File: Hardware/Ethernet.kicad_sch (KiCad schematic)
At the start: 37 parts, among them J1 Conn_01x07_Male, J2 Conn_01x04_Male, J3 Conn_01x02_Male, J4 Conn_01x02_Male, J5 Conn_01x02_Male, J6 Conn_01x02_Male, J7 Conn_01x08_Male, J9 QWIIC_Stackable, U1 W5500, Y1 25.000MHz

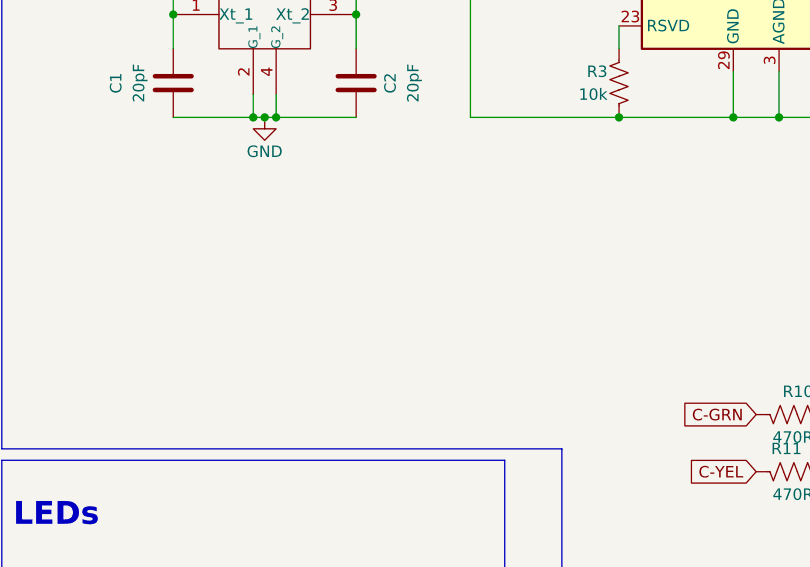
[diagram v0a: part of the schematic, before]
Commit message: More on POE...
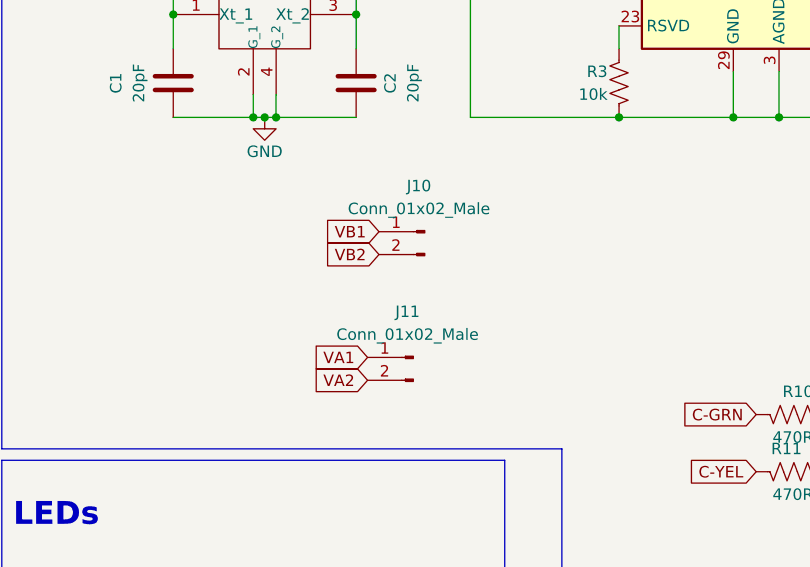
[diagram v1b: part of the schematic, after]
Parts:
- added J10, J11: Conn_01x02_Male, Connector_PinSocket_1.27mm:PinSocket_1x02_P1.27mm_Vertical_SMD_Pin1Right, symbol Connector:Conn_01x02_Male
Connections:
- net VA1: now also J11.1 (Pin_1)
- net VA2: now also J11.2 (Pin_2)
- net VB1: now also J10.1 (Pin_1)
- net VB2: now also J10.2 (Pin_2)
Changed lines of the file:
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@@
+    )
+  )
+  (global_label "VB2" (shape input) (at 157.48 128.27 180) (fields_autoplaced)
+    (effects (font (size 1.27 1.27)) (justify right))
+    (property "Intersheet References" "${INTERSHEET_REFS}" (id 0) (at 151.4988 128.1906 0)
+      (effects (font (size 1.27 1.27)) (justify right) hide)
     )
   )
@@
     )
   )
+  (global_label "VA1" (shape input) (at 156.21 139.7 180) (fields_autoplaced)
+    (effects (font (size 1.27 1.27)) (justify right))
+    (property "Intersheet References" "${INTERSHEET_REFS}" (id 0) (at 150.4102 139.6206 0)
+      (effects (font (size 1.27 1.27)) (justify right) hide)
+    )
+  )
   (global_label "RD+" (shape input) (at 260.35 148.59 0) (fields_autoplaced)
     (effects (font (size 1.27 1.27)) (justify left))
     (property "Intersheet References" "${INTERSHEET_REFS}" (id 0) (at 266.8755 148.5106 0)
       (effects (font (size 1.27 1.27)) (justify left) hide)
+    )
+  )
+  (global_label "VA2" (shape input) (at 156.21 142.24 180) (fields_autoplaced)
+    (effects (font (size 1.27 1.27)) (justify right))
+    (property "Intersheet References" "${INTERSHEET_REFS}" (id 0) (at 150.4102 142.1606 0)
+      (effects (font (size 1.27 1.27)) (justify right) hide)
     )
   )
@@
     (property "Intersheet References" "${INTERSHEET_REFS}" (id 0) (at 268.8107 72.3106 0)
       (effects (font (size 1.27 1.27)) (justify left) hide)
+    )
+  )
+  (global_label "VB1" (shape input) (at 157.48 125.73 180) (fields_autoplaced)
+    (effects (font (size 1.27 1.27)) (justify right))
+    (property "Intersheet References" "${INTERSHEET_REFS}" (id 0) (at 151.4988 125.6506 0)
+      (effects (font (size 1.27 1.27)) (justify right) hide)
     )
   )
@@
     (property "Type" "Tantalum" (id 5) (at 193.04 33.02 0))
     (property "LCSC" "C127946" (id 4) (at 199.39 33.02 0)
+      (effects (font (size 1.27 1.27)) hide)
+    )
+    (pin "1")
+    (pin "2")
+  )
+  (symbol (lib_id "Connector:Conn_01x02_Male") (at 161.29 139.7 0) (mirror y) (unit 1)
+    (in_bom no) (on_board yes)
+    (property "Reference" "J11" (id 0) (at 160.655 134.62 0))
+    (property "Value" "Conn_01x02_Male" (id 1) (at 160.655 137.16 0))
+    (property "Footprint" "Connector_PinSocket_1.27mm:PinSocket_1x02_P1.27mm_Vertical_SMD_Pin1Right" (id 2) (at 161.29 139.7 0)
+      (effects (font (size 1.27 1.27)) hide)
+    )
+    (property "Datasheet" "~" (id 3) (at 161.29 139.7 0)
       (effects (font (size 1.27 1.27)) hide)
     )
@@
     (pin "1")
   )
+  (symbol (lib_id "Connector:Conn_01x02_Male") (at 162.56 125.73 0) (mirror y) (unit 1)
+    (in_bom no) (on_board yes)
+    (property "Reference" "J10" (id 0) (at 161.925 120.65 0))
+    (property "Value" "Conn_01x02_Male" (id 1) (at 161.925 123.19 0))
+    (property "Footprint" "Connector_PinSocket_1.27mm:PinSocket_1x02_P1.27mm_Vertical_SMD_Pin1Right" (id 2) (at 162.56 125.73 0)
+      (effects (font (size 1.27 1.27)) hide)
+    )
+    (property "Datasheet" "~" (id 3) (at 162.56 125.73 0)
+      (effects (font (size 1.27 1.27)) hide)
+    )
+    (pin "1")
+    (pin "2")
+  )
   (symbol (lib_id "Connector:Conn_01x07_Male") (at 72.39 35.56 0) (unit 1)
     (in_bom no) (on_board no)
@@
       (reference "J9") (unit 1) (value "QWIIC_Stackable") (footprint "Tinker:QWIIC_Stack_II")
     )
+    (path "/a064da1d-e50b-4d46-9902-76208c1e200e"
+      (reference "J10") (unit 1) (value "Conn_01x02_Male") (footprint "Connector_PinSocket_1.27mm:PinSocket_1x02_P1.27mm_Vertical_SMD_Pin1Right")
+    )
+    (path "/504ed9d0-691d-452d-b516-7f09cf7e2eae"
+      (reference "J11") (unit 1) (value "Conn_01x02_Male") (footprint "Connector_PinSocket_1.27mm:PinSocket_1x02_P1.27mm_Vertical_SMD_Pin1Right")
+    )
     (path "/99ba0a0f-3edd-4786-889d-f6101a6723f5"

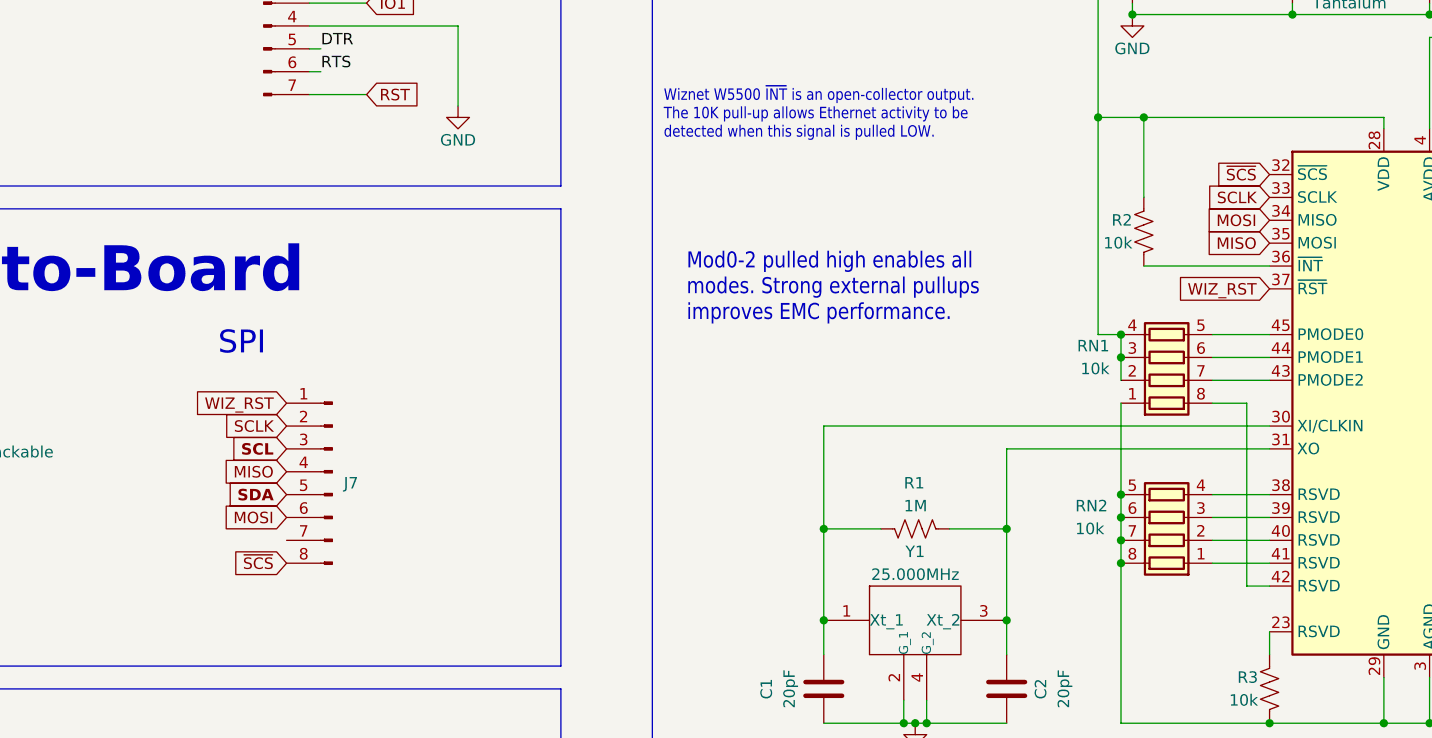
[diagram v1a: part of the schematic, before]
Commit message: Still migrating to 0.2.x
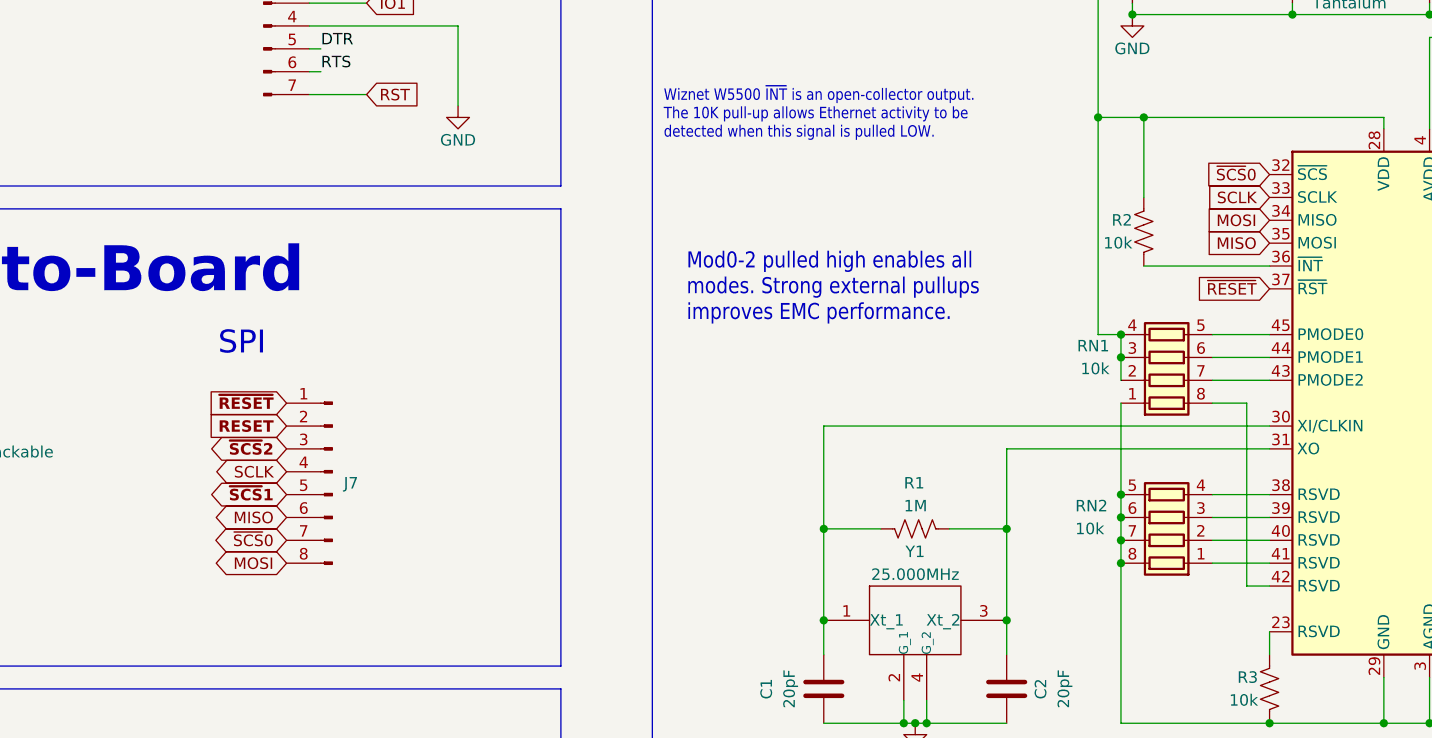
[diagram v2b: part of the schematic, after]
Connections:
- net MISO: now also J7.6 (Pin_6); no longer J7.4 (Pin_4)
- net MOSI: now also J7.8 (Pin_8); no longer J7.6 (Pin_6)
- net SCL: no longer J7.3 (Pin_3)
- net SCLK: now also J7.4 (Pin_4); no longer J7.2 (Pin_2)
- net SDA: no longer J7.5 (Pin_5)
- net ~{SCS}0: now reaches J7.7 (Pin_7)
- net ~{SCS}0: now also U1.32 (~{SCS})
- net WIZ_RST renamed ~{RESET}
- removed net ~{SCS}: J7.8 (Pin_8), U1.32 (~{SCS})
- new net RESET: J7.2 (Pin_2)
- new net ~{SCS}1: J7.5 (Pin_5)
- new net ~{SCS}2: J7.3 (Pin_3)
